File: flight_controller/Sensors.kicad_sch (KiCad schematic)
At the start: 27 parts, among them U10 24LC64-I/SN, U11 FM25V02A-GTR, U12 MPU6500, U13 MS561101BA03-50, U56 ICM-20689, U9 W25Q512JVFIQ

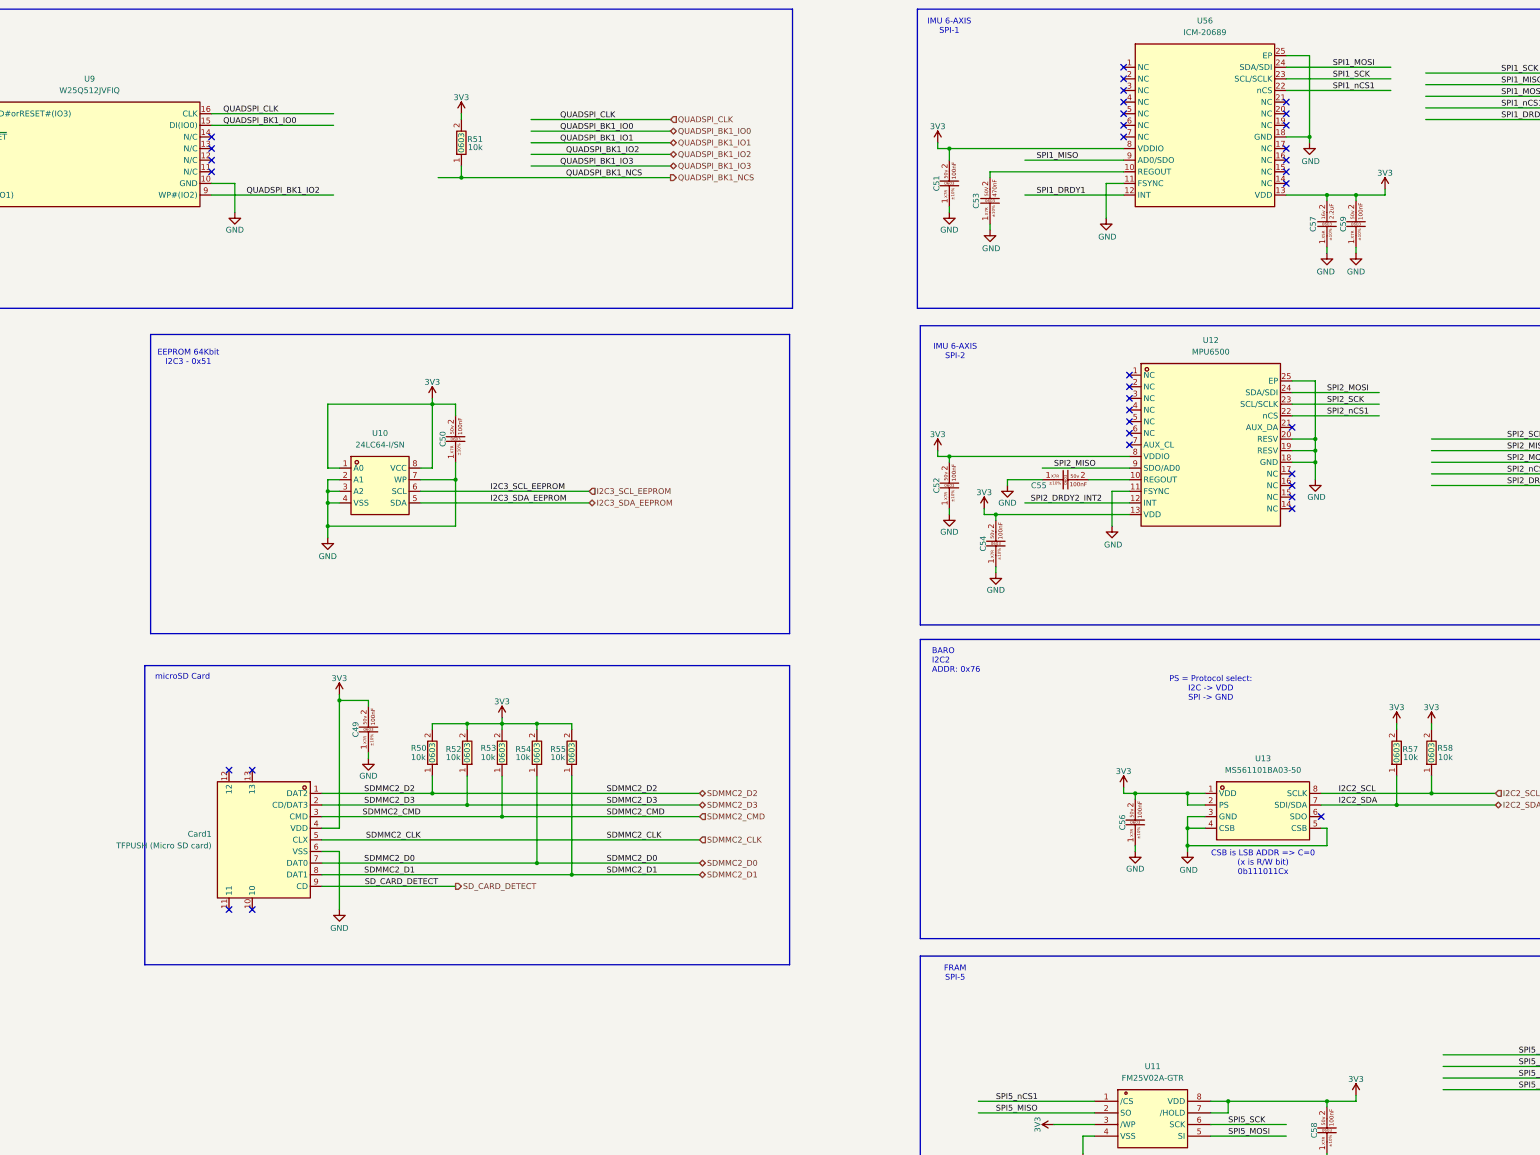
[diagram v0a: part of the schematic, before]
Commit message: Updated power and usb connectors, annotations and netlist check
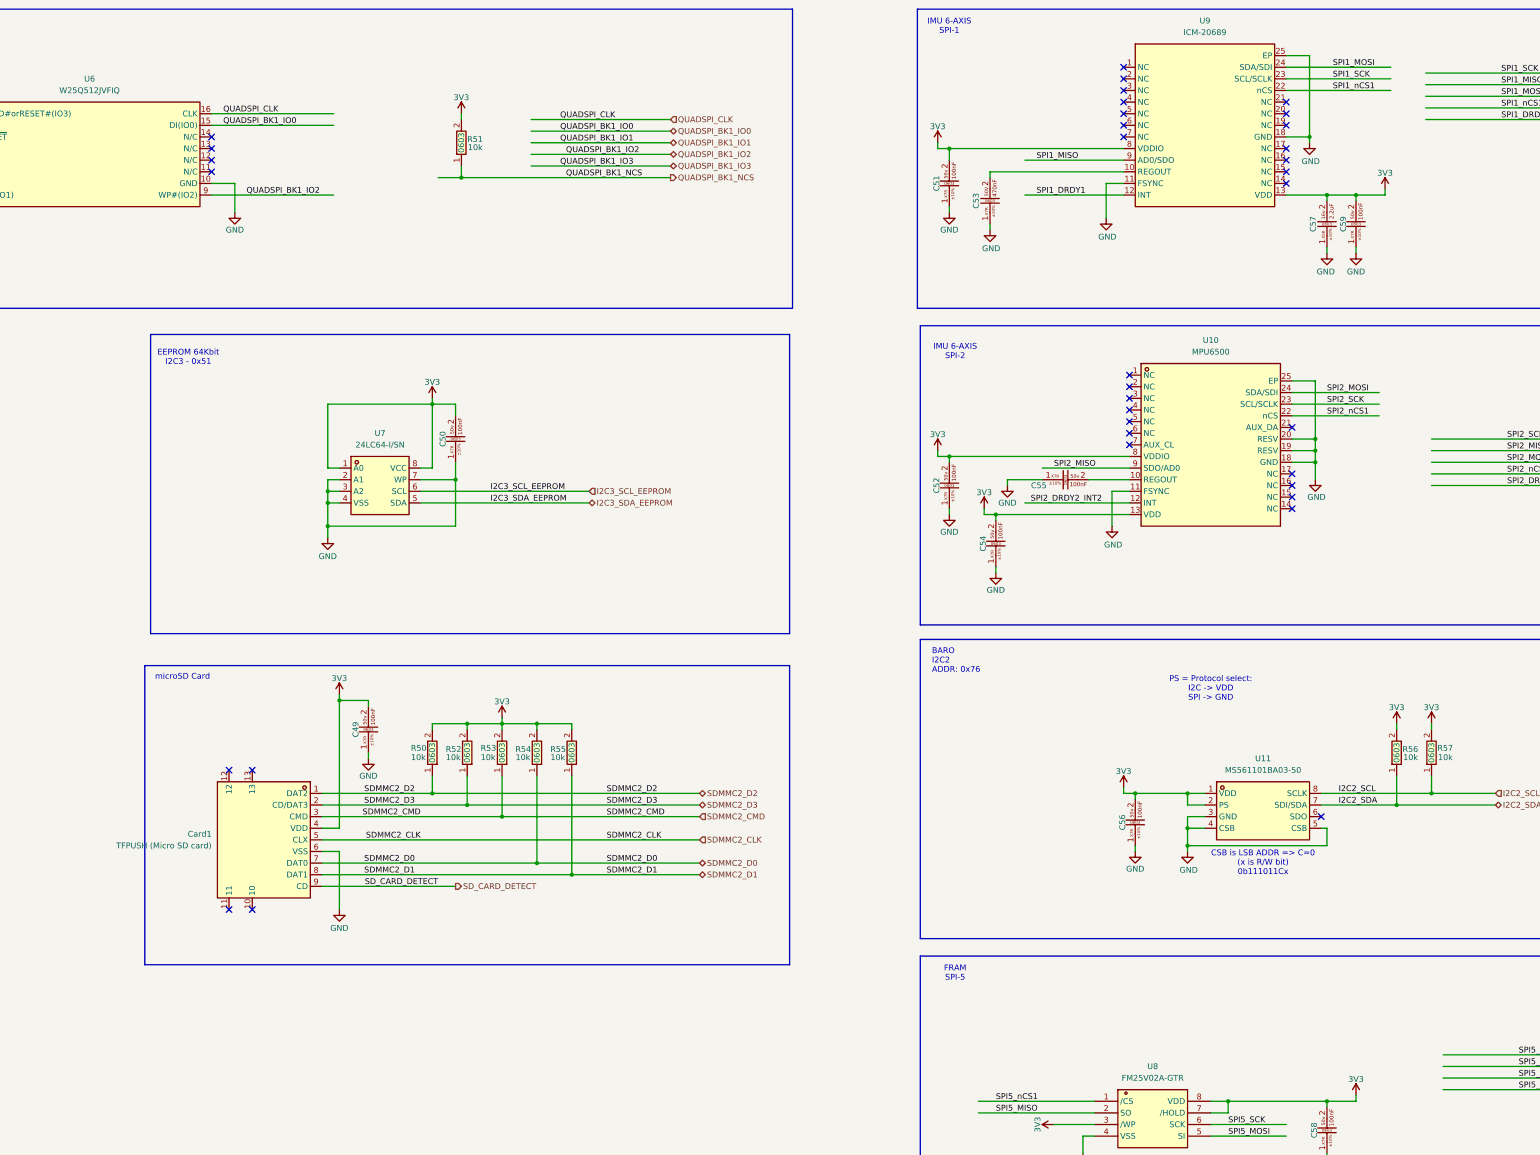
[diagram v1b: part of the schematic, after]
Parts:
- renumbered R57 to R56, R58 to R57, U12 to U10, U13 to U11, U9 to U6, U10 to U7, U11 to U8, U56 to U9

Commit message: Revert to state of commit 2458262 moved all to components to top
Reverts commits: d012532, 3d9c600, 58bc0ac
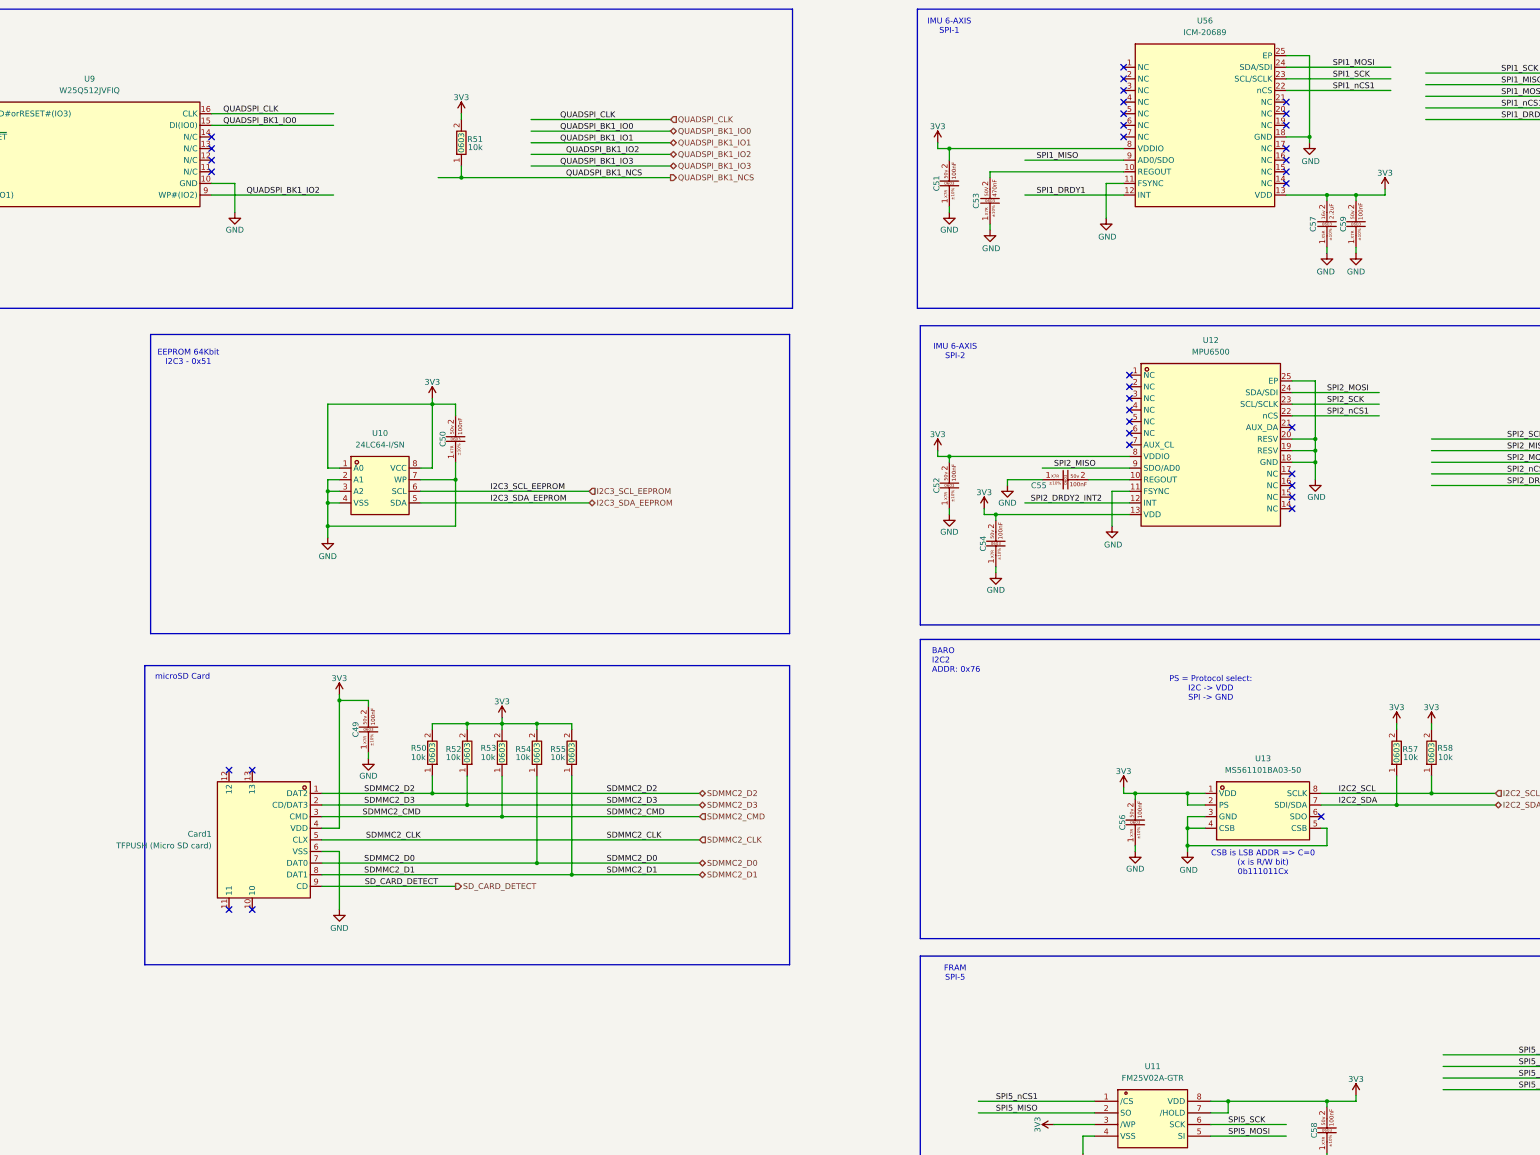
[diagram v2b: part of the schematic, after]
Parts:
- renumbered R56 to R57, R57 to R58, U7 to U10, U8 to U11, U10 to U12, U11 to U13, U9 to U56, U6 to U9
